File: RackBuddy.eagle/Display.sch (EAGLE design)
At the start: 18 parts, among them IC1 ATmega328, IC2 UDN2981A, IC3 4022N, Q1 16MHz

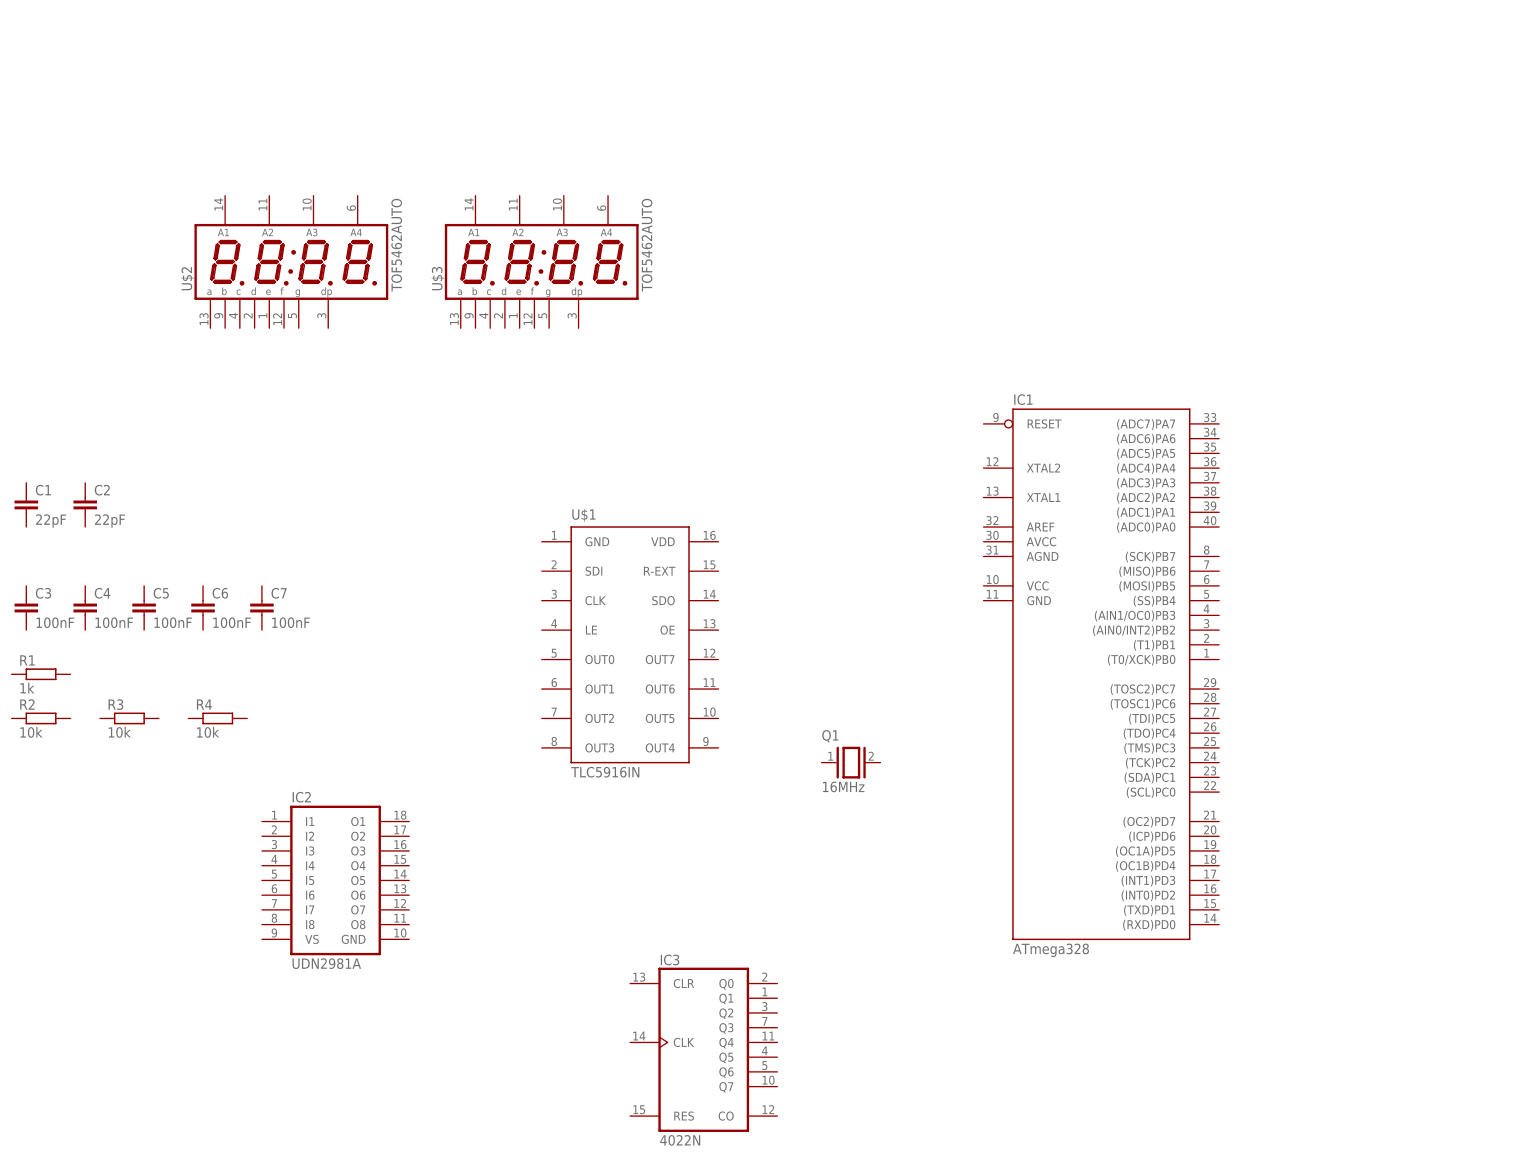
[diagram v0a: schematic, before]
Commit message: Added README
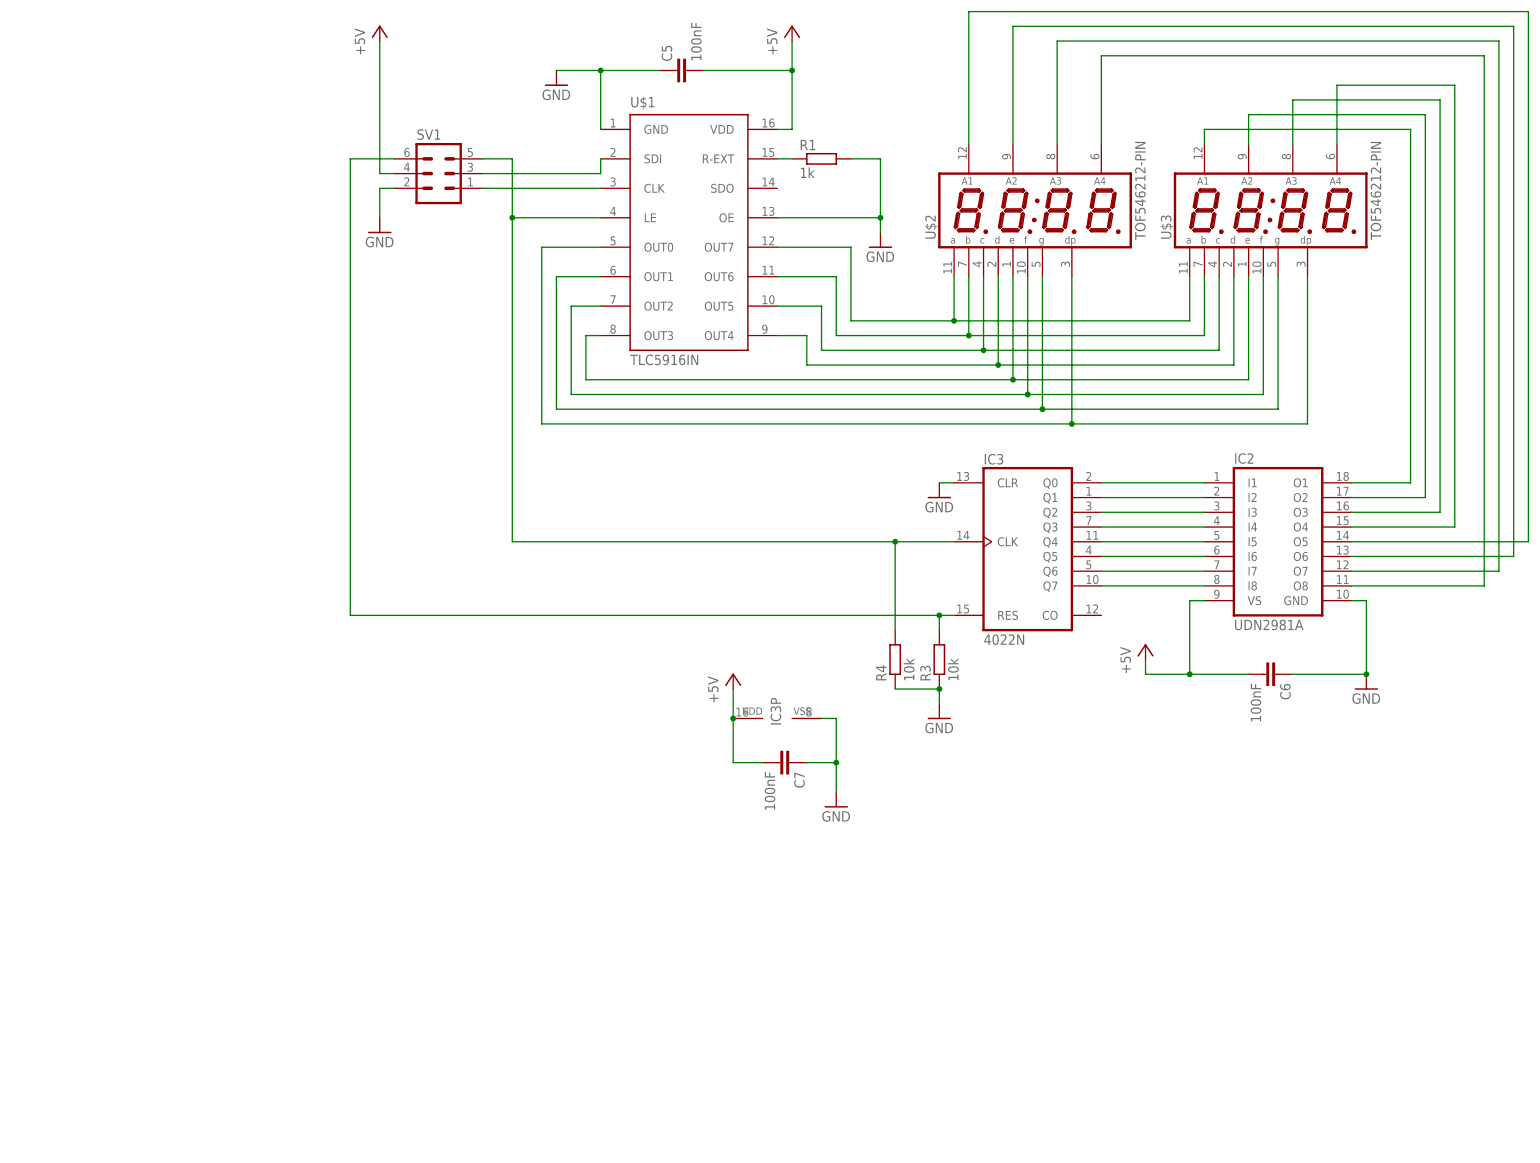
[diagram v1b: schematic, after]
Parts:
- removed C1, C2: 22pF, rcl:C-EU025-024X044
- removed C3, C4: 100nF, rcl:C-EU025-024X044
- removed IC1: ATmega328, avr-7:MEGA32-P
- removed Q1: 16MHz, special:XTAL/S
- removed R2: 10k, rcl:R-EU_0204/7
- added SV1: (no value), con-harting-ml:ML6L
- R3, R4: device rcl:R-EU_0204/7 -> rcl:R-EU_0204/2V
- U$2, U$3: value TOF5462AUTO -> TOF546212-PIN; device TOF5462:TOF5462AUTO -> TOF5462:TOF546212-PIN
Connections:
- new net +5V: C5.2, C6.2, C7.2, IC2.VS, IC3P.VDD, SV1.4, U$1.VDD
- new net CLOCK: SV1.1, U$1.CLK
- new net DATA: SV1.3, U$1.SDI
- new net GND: C5.1, C6.1, C7.1, IC2.GND, IC3A.CLR, IC3P.VSS, R1.2, R3.1, R4.1, SV1.2, U$1.GND, U$1.OE
- new net LATCH: IC3A.CLK, R4.2, SV1.5, U$1.LE
- new net N$1: U$1.OUT6, U$2.B, U$3.B
- new net N$10: IC2.I1, IC3A.Q0
- new net N$11: IC2.I2, IC3A.Q1
- new net N$12: IC2.I3, IC3A.Q2
- new net N$13: IC2.I4, IC3A.Q3
- new net N$14: IC2.I5, IC3A.Q4
- new net N$15: IC2.I6, IC3A.Q5
- new net N$16: IC2.I7, IC3A.Q6
- new net N$17: IC2.I8, IC3A.Q7
- new net N$18: IC2.O1, U$3.A1
- new net N$19: IC2.O5, U$2.A1
- new net N$2: IC2.O2, U$3.A2
- new net N$20: U$1.OUT7, U$2.A, U$3.A
- new net N$21: IC2.O6, U$2.A2
- new net N$22: IC2.O3, U$3.A3
- new net N$23: IC2.O7, U$2.A3
- new net N$24: IC2.O4, U$3.A4
- new net N$25: IC2.O8, U$2.A4
- new net N$3: U$1.OUT5, U$2.C, U$3.C
- new net N$4: U$1.OUT4, U$2.D, U$3.D
- new net N$5: R1.1, U$1.R-EXT
- new net N$6: U$1.OUT3, U$2.E, U$3.E
- new net N$7: U$1.OUT2, U$2.F, U$3.F
- new net N$8: U$1.OUT1, U$2.G, U$3.G
- new net N$9: U$1.OUT0, U$2.DP, U$3.DP
- new net RESET: IC3A.RES, R3.2, SV1.6
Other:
- moved on the sheet: C5, C6, C7, IC2, IC3, R1, R3, R4, U$1, U$2, U$3
